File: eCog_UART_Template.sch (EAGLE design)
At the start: 1 part

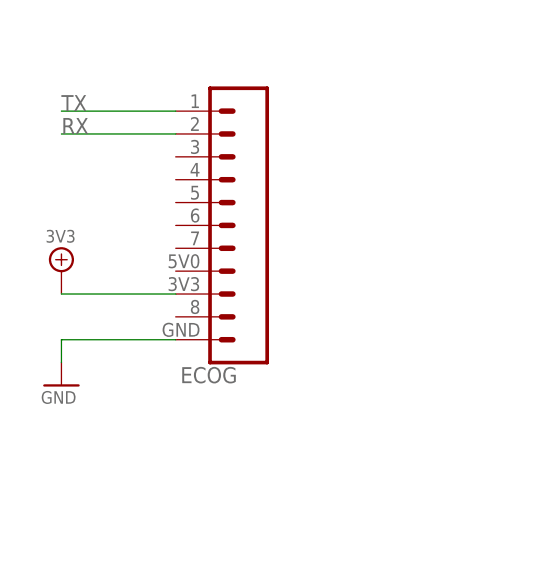
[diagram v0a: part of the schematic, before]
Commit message: Latest updated to V1.4
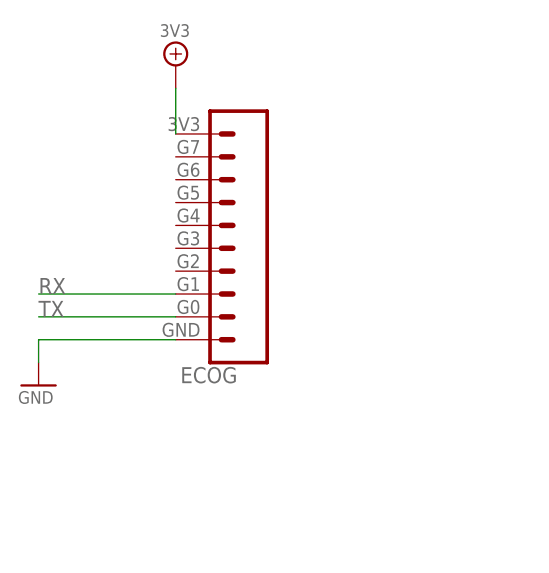
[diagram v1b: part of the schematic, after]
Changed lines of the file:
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@@
 <layer number="54" name="bGND_GNDA" color="1" fill="9" visible="no" active="no"/>
 <layer number="56" name="wert" color="3" fill="1" visible="no" active="no"/>
+<layer number="57" name="tCAD" color="7" fill="1" visible="no" active="no"/>
+<layer number="59" name="tCarbon" color="7" fill="1" visible="no" active="no"/>
+<layer number="60" name="bCarbon" color="7" fill="1" visible="no" active="no"/>
+<layer number="90" name="Modules" color="7" fill="1" visible="yes" active="yes"/>
 <layer number="91" name="Nets" color="2" fill="1" visible="yes" active="yes"/>
 <layer number="92" name="Busses" color="1" fill="1" visible="yes" active="yes"/>
@@
 <layer number="97" name="Info" color="7" fill="1" visible="yes" active="yes"/>
 <layer number="98" name="Guide" color="6" fill="1" visible="yes" active="yes"/>
+<layer number="99" name="SpiceOrder" color="7" fill="1" visible="no" active="no"/>
 <layer number="100" name="Muster" color="7" fill="1" visible="no" active="no"/>
 <layer number="101" name="Patch_Top" color="12" fill="4" visible="no" active="yes"/>
@@
 <layer number="111" name="tGTest" color="7" fill="1" visible="yes" active="yes"/>
 <layer number="112" name="bGTest" color="7" fill="1" visible="yes" active="yes"/>
+<layer number="113" name="ReferenceLS" color="7" fill="1" visible="no" active="no"/>
 <layer number="116" name="Patch_BOT" color="9" fill="4" visible="no" active="yes"/>
+<layer number="118" name="Rect_Pads" color="7" fill="1" visible="no" active="no"/>
 <layer number="121" name="_tsilk" color="7" fill="1" visible="yes" active="yes"/>
 <layer number="122" name="_bsilk" color="7" fill="1" visible="no" active="yes"/>
@@
 <layer number="124" name="bTestmark" color="7" fill="1" visible="yes" active="yes"/>
 <layer number="125" name="_tNames" color="7" fill="1" visible="yes" active="yes"/>
+<layer number="126" name="_bNames" color="7" fill="1" visible="yes" active="yes"/>
+<layer number="127" name="_tValues" color="7" fill="1" visible="yes" active="yes"/>
+<layer number="128" name="_bValues" color="7" fill="1" visible="yes" active="yes"/>
+<layer number="129" name="Mask" color="7" fill="1" visible="yes" active="yes"/>
 <layer number="131" name="prix" color="7" fill="1" visible="no" active="yes"/>
 <layer number="132" name="test" color="7" fill="1" visible="no" active="yes"/>
@@
 <layer number="135" name="Port3" color="7" fill="1" visible="yes" active="yes"/>
 <layer number="144" name="Drill_legend" color="7" fill="1" visible="yes" active="yes"/>
+<layer number="150" name="Notes" color="7" fill="1" visible="yes" active="yes"/>
 <layer number="151" name="HeatSink" color="7" fill="1" visible="no" active="yes"/>
+<layer number="152" name="_bDocu" color="7" fill="1" visible="yes" active="yes"/>
+<layer number="153" name="FabDoc1" color="6" fill="1" visible="no" active="no"/>
+<layer number="154" name="FabDoc2" color="2" fill="1" visible="no" active="no"/>
+<layer number="155" name="FabDoc3" color="7" fill="15" visible="no" active="no"/>
 <layer number="199" name="Contour" color="7" fill="1" visible="yes" active="yes"/>
 <layer number="200" name="200bmp" color="1" fill="10" visible="no" active="no"/>
@@
 <layer number="223" name="223bmp" color="24" fill="1" visible="no" active="no"/>
 <layer number="224" name="224bmp" color="25" fill="1" visible="no" active="no"/>
+<layer number="225" name="225bmp" color="7" fill="1" visible="yes" active="yes"/>
+<layer number="226" name="226bmp" color="7" fill="1" visible="yes" active="yes"/>
+<layer number="227" name="227bmp" color="7" fill="1" visible="yes" active="yes"/>
+<layer number="228" name="228bmp" color="7" fill="1" visible="yes" active="yes"/>
+<layer number="229" name="229bmp" color="7" fill="1" visible="yes" active="yes"/>
+<layer number="230" name="230bmp" color="7" fill="1" visible="yes" active="yes"/>
+<layer number="231" name="Eagle3D_PG1" color="7" fill="1" visible="no" active="no"/>
+<layer number="232" name="Eagle3D_PG2" color="7" fill="1" visible="no" active="no"/>
+<layer number="233" name="Eagle3D_PG3" color="7" fill="1" visible="no" active="no"/>
+<layer number="248" name="Housing" color="7" fill="1" visible="yes" active="yes"/>
+<layer number="249" name="Edge" color="7" fill="1" visible="yes" active="yes"/>
 <layer number="250" name="Descript" color="3" fill="1" visible="no" active="no"/>
 <layer number="251" name="SMDround" color="4" fill="9" visible="no" active="yes"/>
 <layer number="254" name="cooling" color="7" fill="1" visible="no" active="yes"/>
+<layer number="255" name="routoute" color="7" fill="1" visible="yes" active="yes"/>
 </layers>
 <schematic xreflabel="%F%N/%S.%C%R" xrefpart="/%S.%C%R">
@@
 <instance part="FRAME1" gate="G$1" x="0" y="0"/>
 <instance part="ECOG" gate="ECOG_GENERAL" x="55.88" y="53.34"/>
-<instance part="3V3_PWR1" gate="A" x="38.1" y="63.5"/>
-<instance part="GND1" gate="A" x="38.1" y="50.8"/>
+<instance part="3V3_PWR1" gate="A" x="50.8" y="86.36"/>
+<instance part="GND1" gate="A" x="35.56" y="50.8"/>
 </instances>
 <busses>
 </busses>
 <nets>
-<net name="TX" class="0">
-<segment>
-<pinref part="ECOG" gate="ECOG_GENERAL" pin="G0"/>
-<wire x1="50.8" y1="81.28" x2="38.1" y2="81.28" width="0.2032" layer="91"/>
-<label x="38.1" y="81.28" size="1.778" layer="95"/>
-</segment>
-</net>
-<net name="RX" class="0">
-<segment>
-<pinref part="ECOG" gate="ECOG_GENERAL" pin="G1"/>
-<wire x1="50.8" y1="78.74" x2="38.1" y2="78.74" width="0.2032" layer="91"/>
-<label x="38.1" y="78.74" size="1.778" layer="95"/>
-</segment>
-</net>
 <net name="3V3" class="0">
 <segment>
 <pinref part="ECOG" gate="ECOG_GENERAL" pin="3V3"/>
 <pinref part="3V3_PWR1" gate="A" pin="3V3"/>
-<wire x1="50.8" y1="60.96" x2="38.1" y2="60.96" width="0.2032" layer="91"/>
+<wire x1="50.8" y1="78.74" x2="50.8" y2="83.82" width="0.2032" layer="91"/>
 </segment>
 </net>
@@
 <pinref part="ECOG" gate="ECOG_GENERAL" pin="GND"/>
 <pinref part="GND1" gate="A" pin="GND"/>
-<wire x1="50.8" y1="55.88" x2="38.1" y2="55.88" width="0.2032" layer="91"/>
-<wire x1="38.1" y1="55.88" x2="38.1" y2="53.34" width="0.2032" layer="91"/>
+<wire x1="50.8" y1="55.88" x2="35.56" y2="55.88" width="0.2032" layer="91"/>
+<wire x1="35.56" y1="55.88" x2="35.56" y2="53.34" width="0.2032" layer="91"/>
 </segment>
 </net>
+<net name="TX" class="0">
+<segment>
+<pinref part="ECOG" gate="ECOG_GENERAL" pin="G0"/>
+<wire x1="50.8" y1="58.42" x2="35.56" y2="58.42" width="0.2032" layer="91"/>
+<label x="35.56" y="58.42" size="1.778" layer="95"/>
+</segment>
+</net>
+<net name="RX" class="0">
+<segment>
+<pinref part="ECOG" gate="ECOG_GENERAL" pin="G1"/>
+<wire x1="50.8" y1="60.96" x2="35.56" y2="60.96" width="0.2032" layer="91"/>
+<label x="35.56" y="60.96" size="1.778" layer="95"/>
+</segment>
+</net>
